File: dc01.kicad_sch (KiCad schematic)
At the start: 76 parts, among them J1 USB_C_Receptacle_USB2.0, J2 PROG/DEBUG, J3 Conn_01x06, J4 RJ12, J5 RJ12, J6 Screw_Terminal_01x02, J7 Screw_Terminal_01x02, J8 Conn_01x02, U1 STM32F103C8Tx, U2 AMS1117-3.3, U3 ADM2483xRW, U4 ADUM1250, U6 LM78M05_TO252, U7 INA219AxDCN, Y1 8 MHz

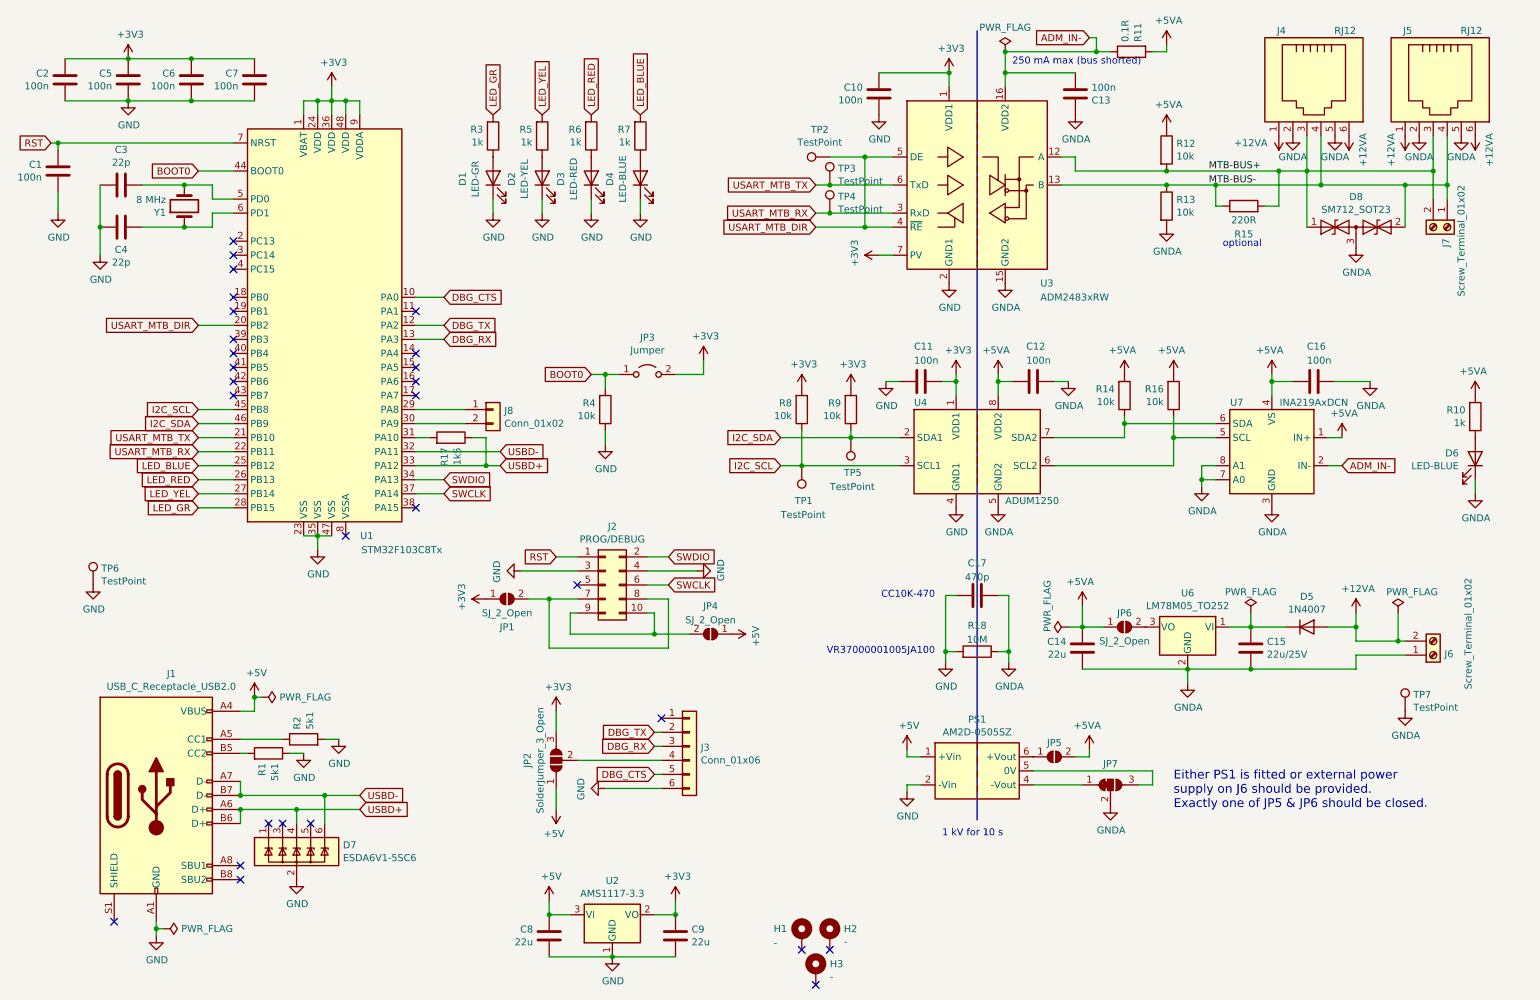
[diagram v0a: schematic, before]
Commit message: Remove unused parts.
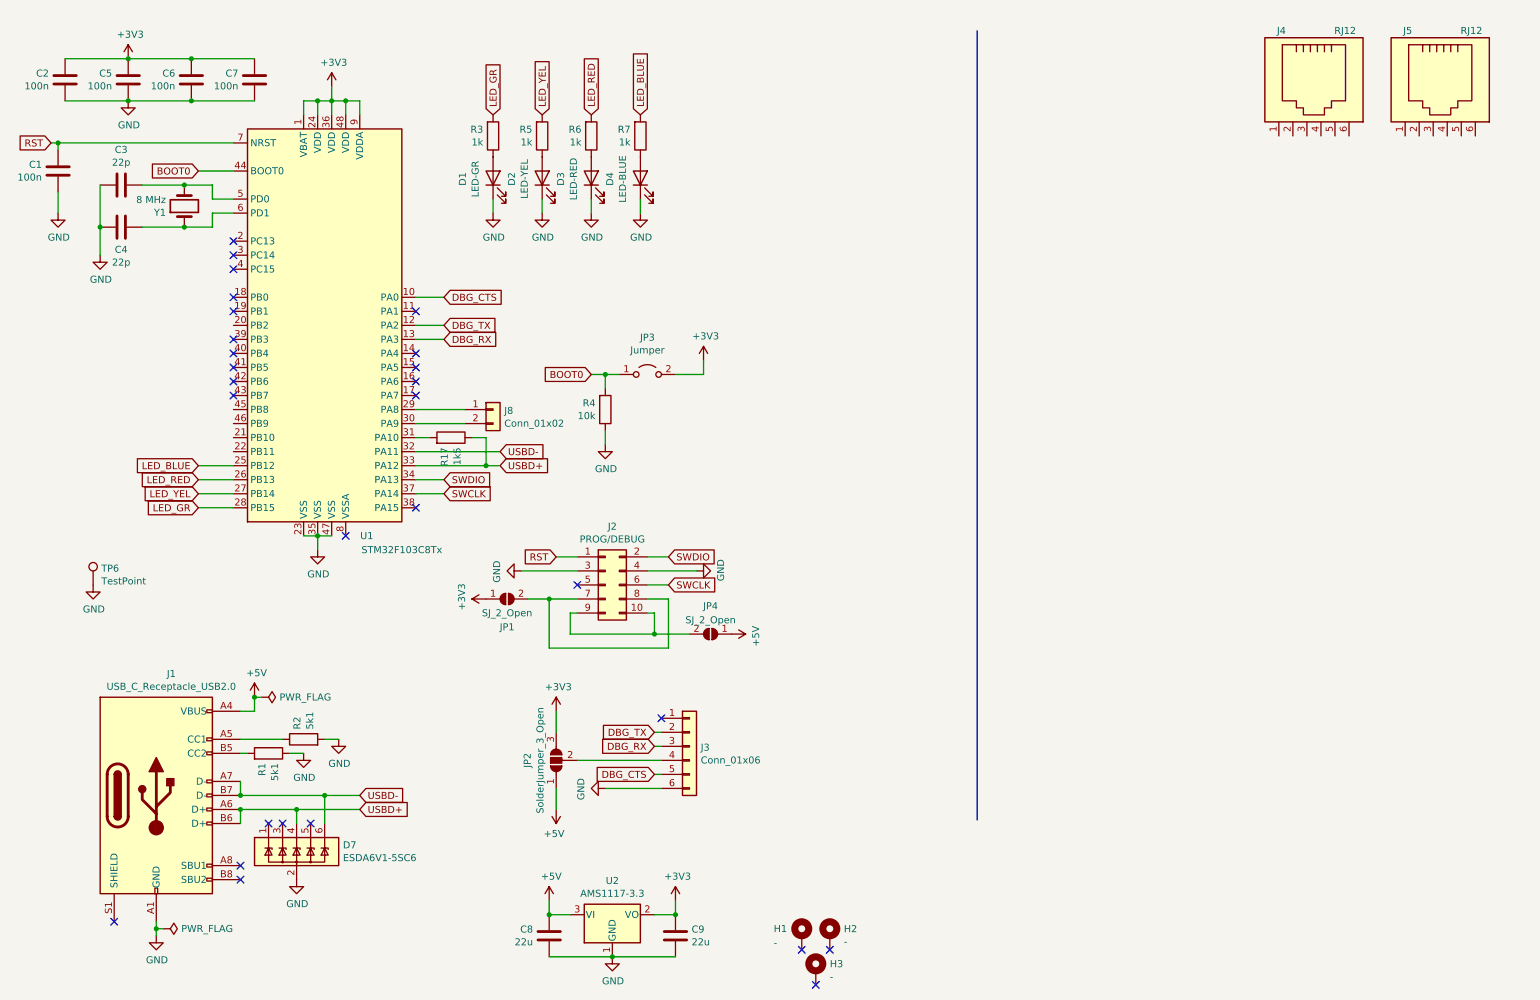
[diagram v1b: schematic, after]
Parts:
- removed C10, C11, C12, C13, C16: 100n, Capacitor_SMD:C_0805_2012Metric, symbol Device:C
- removed C14: 22u, Capacitor_SMD:C_0805_2012Metric, symbol Device:C
- removed C15: 22u/25V, Capacitor_SMD:C_0805_2012Metric, symbol Device:C
- removed C17: 470p, Capacitor_THT:C_Disc_D12.5mm_W5.0mm_P10.00mm, symbol Device:C
- removed D5: 1N4007, Diode_SMD:D_SOD-123, symbol Device:D
- removed D6: LED-BLUE, LED_SMD:LED_0805_2012Metric, symbol Device:LED
- removed D8: SM712_SOT23, Package_TO_SOT_SMD:SOT-23, symbol Diode:SM712_SOT23
- removed J6, J7: Screw_Terminal_01x02, TerminalBlock_4Ucon:TerminalBlock_4Ucon_1x02_P3.50mm_Horizontal, symbol Connector:Screw_Terminal_01x02
- removed JP5, JP6: SJ_2_Open, Jumper:SolderJumper-2_P1.3mm_Open_RoundedPad1.0x1.5mm, symbol Jumper:SolderJumper_2_Open
- removed JP7: SJ3_Bridged12, Jumper:SolderJumper-3_P1.3mm_Bridged12_RoundedPad1.0x1.5mm_NumberLabels, symbol Jumper:SolderJumper_3_Bridged12
- removed PS1: AM2D-0505SZ, Converter_DCDC:Converter_DCDC_XP_POWER-IHxxxxS_THT, symbol Converter_DCDC:IH0505S
- removed R10: 1k, Resistor_SMD:R_0805_2012Metric, symbol Device:R
- removed R11: 0.1R, Resistor_SMD:R_1206_3216Metric, symbol Device:R
- removed R12, R13, R14, R16, R8, R9: 10k, Resistor_SMD:R_0805_2012Metric, symbol Device:R
- removed R15: 220R, Resistor_SMD:R_0805_2012Metric, symbol Device:R
- removed R18: 10M, Resistor_THT:R_Axial_DIN0207_L6.3mm_D2.5mm_P10.16mm_Horizontal, symbol Device:R
- removed TP1, TP2, TP3, TP4, TP5: TestPoint, TestPoint:TestPoint_Pad_D1.0mm, symbol Connector:TestPoint
- removed TP7: TestPoint, TestPoint:TestPoint_Loop_D3.50mm_Drill1.4mm_Beaded, symbol Connector:TestPoint
- removed U3: ADM2483xRW, Package_SO:SOIC-16W_7.5x10.3mm_P1.27mm, symbol Interface_UART:ADM2483xRW
- removed U4: ADUM1250, Package_SO:SO-8_3.9x4.9mm_P1.27mm, symbol Interface_I2C:ADUM1250
- removed U6: LM78M05_TO252, Package_TO_SOT_SMD:TO-252-2, symbol Regulator_Linear:LM78M05_TO252
- removed U7: INA219AxDCN, Package_TO_SOT_SMD:SOT-23-8, symbol Analog_ADC:INA219AxDCN
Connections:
- removed net +12VA: J4.1, J4.6, J5.1, J5.6
- removed net GNDA: J4.2, J4.5, J5.2, J5.5
- net I2C_SCL: no longer names the net of U1.45 (PB8)
- net I2C_SDA: no longer names the net of U1.46 (PB9)
- net MTB-BUS+: no longer names the net of J5.3
- net MTB-BUS+: no longer J4.3
- net MTB-BUS-: no longer names the net of J5.4
- net MTB-BUS-: no longer J4.4
- net USART_MTB_DIR: no longer names the net of U1.20 (PB2)
- net USART_MTB_RX: no longer names the net of U1.22 (PB11)
- net USART_MTB_TX: no longer names the net of U1.21 (PB10)
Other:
- note removed: "1 kV for 10 s"
- note removed: "250 mA max (bus shorted)"
- note removed: "CC10K-470"
- note removed: "Either PS1 is fitted or external power supply on J6 should be provided. Exactly one of JP5 & JP6 should be closed."
- note removed: "VR37000001005JA100"
- note removed: "optional"
- title: MTB-USB v4 -> DCC cutter DC-01

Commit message: Add & wire relay part.
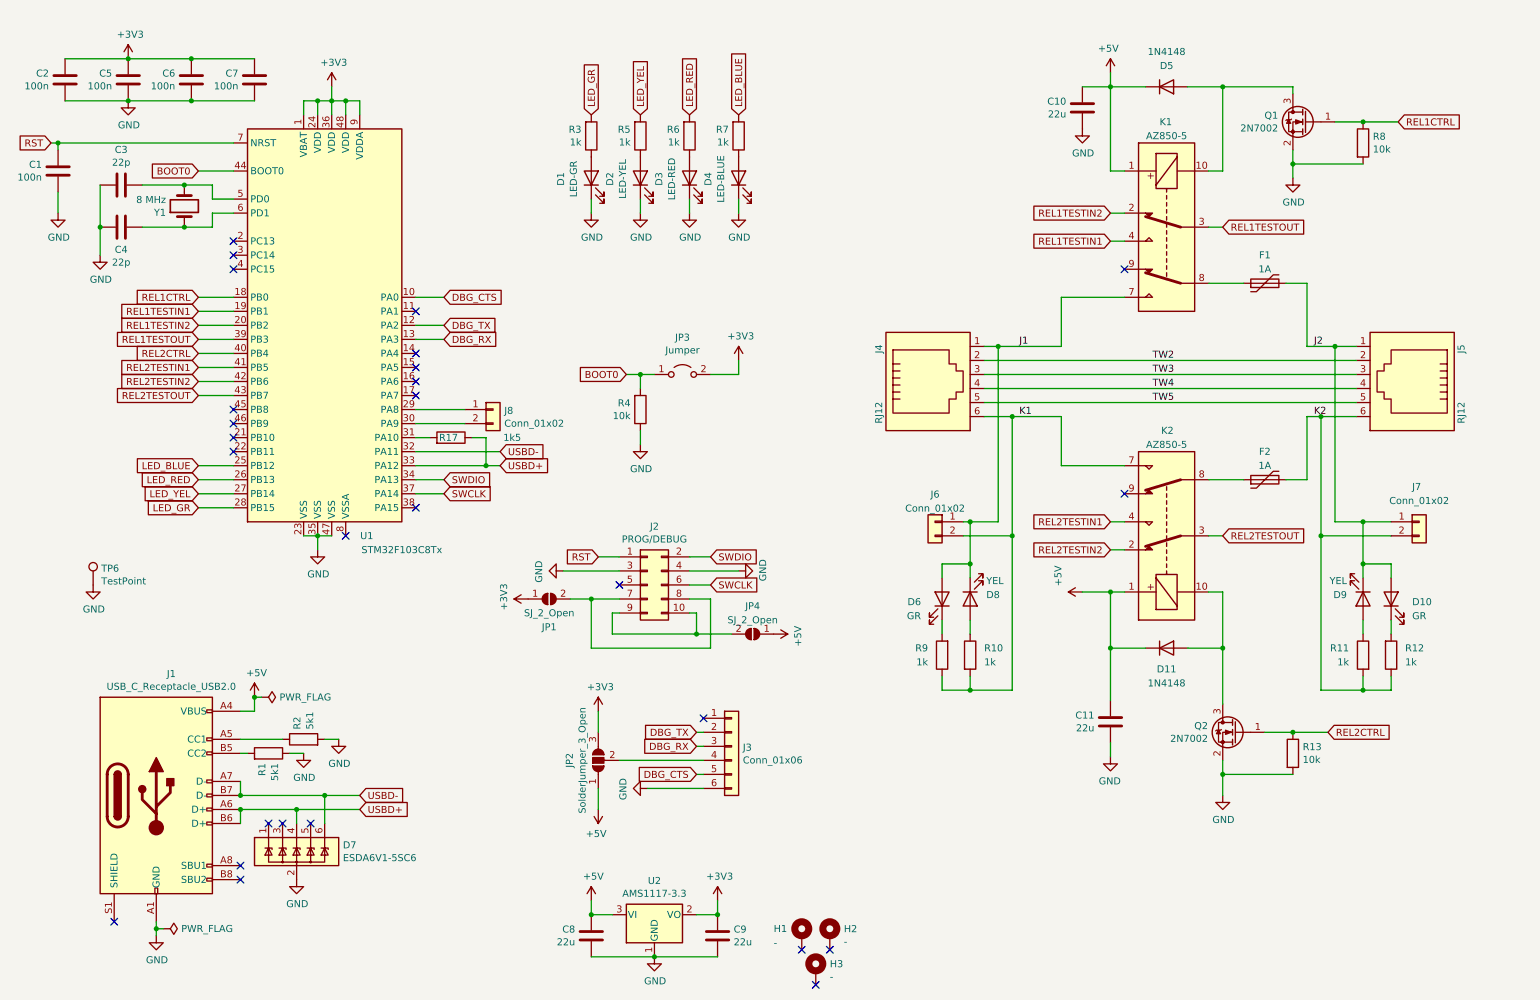
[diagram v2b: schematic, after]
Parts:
- added C10, C11: 22u, Capacitor_SMD:C_0805_2012Metric, symbol Device:C
- added D10, D6: GR, symbol Device:LED
- added D11, D5: 1N4148, Diode_THT:D_DO-35_SOD27_P7.62mm_Horizontal, symbol Diode:1N4148
- added D8, D9: YEL, symbol Device:LED
- added F1, F2: 1A, symbol Device:Polyfuse
- added J6, J7: Conn_01x02, symbol Connector_Generic:Conn_01x02
- added K1, K2: AZ850-5, Relay_THT:Relay_DPDT_FRT5, symbol Relay:AZ850-x
- added Q1, Q2: 2N7002, Package_TO_SOT_SMD:SOT-23, symbol Transistor_FET:2N7002
- added R10, R11, R12, R9: 1k, symbol Device:R
- added R13, R8: 10k, Resistor_SMD:R_0805_2012Metric_Pad1.20x1.40mm_HandSolder, symbol Device:R
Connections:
- net +5V: now also C10.1, C11.1, D11.1 (K), D5.1 (K), K1.1, K2.1
- net GND: now also C10.2, C11.2, Q1.2 (S), Q2.2 (S), R13.2, R8.2
- net J2: now reaches J5.1
- net J2: now also D10.2 (A), D9.1 (K), F1.2, J7.1 (Pin_1)
- net TW2: now reaches J5.2
- net TW2: now also J4.2
- net TW3: now reaches J5.3
- net TW3: now also J4.3
- net TW4: now reaches J5.4
- net TW4: now also J4.4
- net TW5: now reaches J5.5
- net TW5: now also J4.5
- net K2: now reaches J5.6
- net K2: now also F2.2, J7.2 (Pin_2), R11.2, R12.1
- net J1: now reaches J4.1
- net J1: now also D6.2 (A), D8.1 (K), J6.1 (Pin_1), K1.7
- net K1: now reaches J4.6
- net K1: now also J6.2 (Pin_2), K2.7, R10.2, R9.1
- net REL1CTRL: now reaches U1.18 (PB0)
- net REL1CTRL: now also Q1.1 (G), R8.1
- net REL1TESTIN1: now reaches U1.19 (PB1)
- net REL1TESTIN1: now also K1.4
- net REL1TESTIN2: now reaches U1.20 (PB2)
- net REL1TESTIN2: now also K1.2
- net REL1TESTOUT: now reaches U1.39 (PB3)
- net REL1TESTOUT: now also K1.3
- net REL2CTRL: now reaches U1.40 (PB4)
- net REL2CTRL: now also Q2.1 (G), R13.1
- net REL2TESTIN1: now reaches U1.41 (PB5)
- net REL2TESTIN1: now also K2.4
- net REL2TESTIN2: now reaches U1.42 (PB6)
- net REL2TESTIN2: now also K2.2
- net REL2TESTOUT: now reaches U1.43 (PB7)
- net REL2TESTOUT: now also K2.3
- new net: D9.2 (A), R11.1
- new net: D8.2 (A), R10.1
- new net: D5.2 (A), K1.10, Q1.3 (D)
- new net: F1.1, K1.8
- new net: D10.1 (K), R12.2
- new net: D6.1 (K), R9.2
- new net: F2.1, K2.8
- new net: D11.2 (A), K2.10, Q2.3 (D)
- no-connect marks 28 -> 27
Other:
- moved on the sheet: C8, C9, D1, D2, D3, D4, J2, J3, J4, J5, JP1, JP2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
